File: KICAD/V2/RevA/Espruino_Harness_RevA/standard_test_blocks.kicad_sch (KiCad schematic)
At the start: 91 parts, among them J201 EXTERNAL_ANALOG_STIMULUS_0_TO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, J301 GROVE_I2C, J302 MCP23017_GPIO, J401 MCP3008_ANALOGUE_BREAKOUT, J402 PIHUT_MICROSD_BREAKOUT_106696, J501 DS18B20_SENSOR_A, J502 DS18B20_SENSOR_B, J503 2K2_DQ_4K7, J504 DS2413_MODULE, J701 UART_PEER_DIAGNOSTIC, J902 PIXEL_SHIFTER_6066, Q301 2N7002, Q302 2N7002, U301 MCP23017-E/SO, U401 MCP3008, U701 TMUX1511

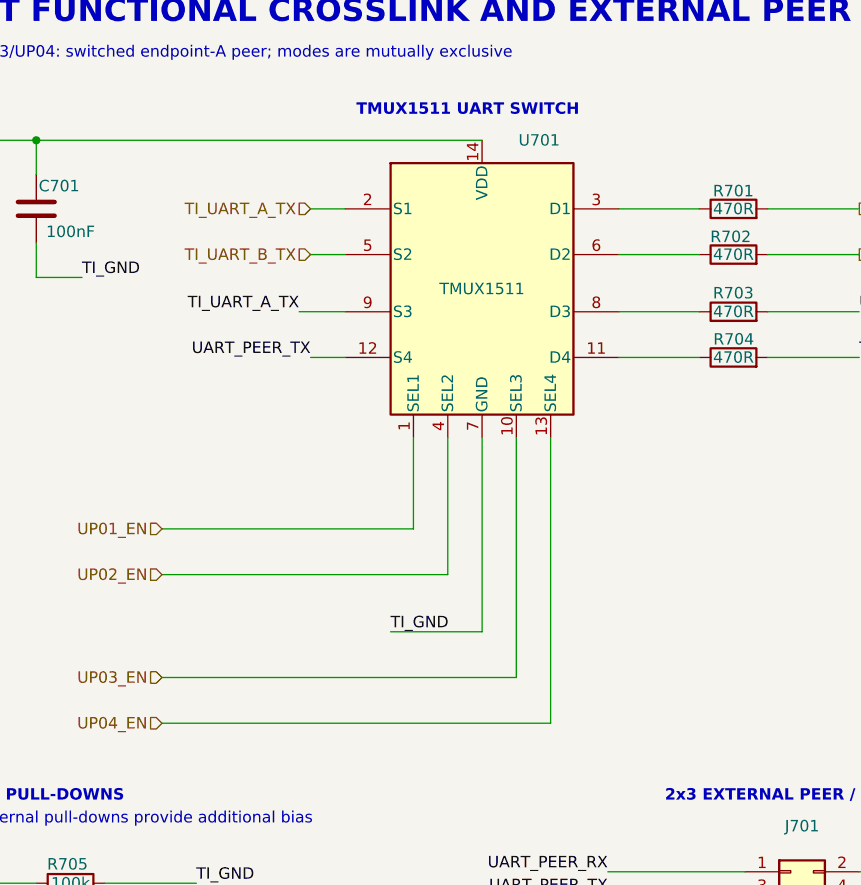
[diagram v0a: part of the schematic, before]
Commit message: Implement V2 routing fabric and control
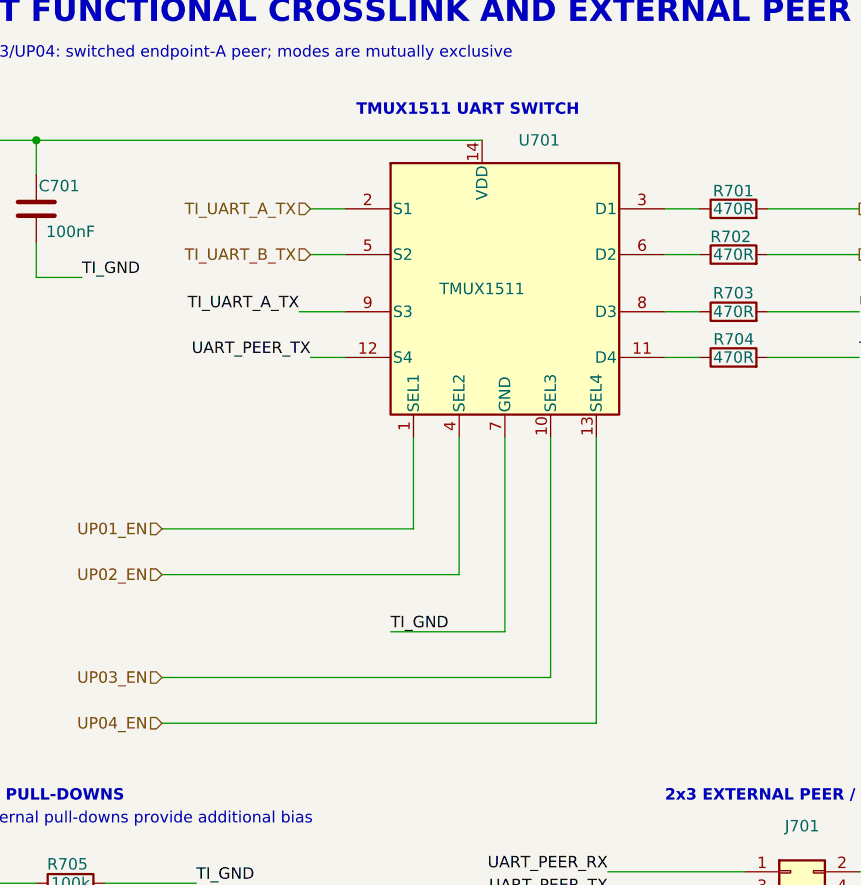
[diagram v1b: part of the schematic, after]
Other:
- moved on the sheet: U701
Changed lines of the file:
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@@
+	(wire
+		(pts
+			(xy 120.65 302.26) (xy 120.65 270.51)
+		)
+		(stroke
+			(width 0)
+			(type default)
+		)
+	)
 	(wire
 		(pts
@@
 	(wire
 		(pts
+			(xy 128.27 245.11) (xy 132.08 245.11)
+		)
+		(stroke
+			(width 0)
+			(type default)
+		)
+	)
+	(wire
+		(pts
 			(xy 514.35 114.3) (xy 514.35 113.03)
 		)
@@
 	(wire
 		(pts
+			(xy 128.27 256.54) (xy 132.08 256.54)
+		)
+		(stroke
+			(width 0)
+			(type default)
+		)
+	)
+	(wire
+		(pts
 			(xy 170.18 201.93) (xy 182.88 201.93)
 		)
@@
 	(wire
 		(pts
-			(xy 107.95 292.1) (xy 97.79 292.1)
+			(xy 110.49 292.1) (xy 97.79 292.1)
 		)
 		(stroke
@@
 	(wire
 		(pts
+			(xy 128.27 261.62) (xy 132.08 261.62)
+		)
+		(stroke
+			(width 0)
+			(type default)
+		)
+	)
+	(wire
+		(pts
 			(xy 38.1 196.85) (xy 86.36 196.85)
 		)
@@
 	(wire
 		(pts
+			(xy 128.27 250.19) (xy 132.08 250.19)
+		)
+		(stroke
+			(width 0)
+			(type default)
+		)
+	)
+	(wire
+		(pts
 			(xy 359.41 43.18) (xy 373.38 43.18)
 		)
@@
 	(wire
 		(pts
-			(xy 123.19 245.11) (xy 132.08 245.11)
-		)
-		(stroke
-			(width 0)
-			(type default)
-		)
-	)
-	(wire
-		(pts
 			(xy 139.7 245.11) (xy 149.86 245.11)
 		)
@@
 	(wire
 		(pts
-			(xy 123.19 250.19) (xy 132.08 250.19)
-		)
-		(stroke
-			(width 0)
-			(type default)
-		)
-	)
-	(wire
-		(pts
 			(xy 139.7 250.19) (xy 149.86 250.19)
 		)
@@
 	(wire
 		(pts
-			(xy 123.19 256.54) (xy 132.08 256.54)
-		)
-		(stroke
-			(width 0)
-			(type default)
-		)
-	)
-	(wire
-		(pts
 			(xy 139.7 256.54) (xy 149.86 256.54)
 		)
@@
 	(wire
 		(pts
-			(xy 123.19 261.62) (xy 132.08 261.62)
-		)
-		(stroke
-			(width 0)
-			(type default)
-		)
-	)
-	(wire
-		(pts
 			(xy 139.7 261.62) (xy 149.86 261.62)
 		)
@@
 	(wire
 		(pts
-			(xy 104.14 270.51) (xy 104.14 285.75)
-		)
-		(stroke
-			(width 0)
-			(type default)
-		)
-	)
-	(wire
-		(pts
-			(xy 72.39 285.75) (xy 104.14 285.75)
-		)
-		(stroke
-			(width 0)
-			(type default)
-		)
-	)
-	(wire
-		(pts
-			(xy 111.76 270.51) (xy 111.76 297.18)
-		)
-		(stroke
-			(width 0)
-			(type default)
-		)
-	)
-	(wire
-		(pts
-			(xy 72.39 297.18) (xy 111.76 297.18)
-		)
-		(stroke
-			(width 0)
-			(type default)
-		)
-	)
-	(wire
-		(pts
-			(xy 115.57 270.51) (xy 115.57 302.26)
-		)
-		(stroke
-			(width 0)
-			(type default)
-		)
-	)
-	(wire
-		(pts
-			(xy 72.39 302.26) (xy 115.57 302.26)
+			(xy 105.41 270.51) (xy 105.41 285.75)
+		)
+		(stroke
+			(width 0)
+			(type default)
+		)
+	)
+	(wire
+		(pts
+			(xy 72.39 285.75) (xy 105.41 285.75)
+		)
+		(stroke
+			(width 0)
+			(type default)
+		)
+	)
+	(wire
+		(pts
+			(xy 115.57 270.51) (xy 115.57 297.18)
+		)
+		(stroke
+			(width 0)
+			(type default)
+		)
+	)
+	(wire
+		(pts
+			(xy 72.39 297.18) (xy 115.57 297.18)
+		)
+		(stroke
+			(width 0)
+			(type default)
+		)
+	)
+	(wire
+		(pts
+			(xy 72.39 302.26) (xy 120.65 302.26)
 		)
 		(stroke
@@
 	(wire
 		(pts
-			(xy 107.95 292.1) (xy 107.95 270.51)
-		)
-		(stroke
+			(xy 110.49 292.1) (xy 110.49 270.51)
+		)
+		(stroke
